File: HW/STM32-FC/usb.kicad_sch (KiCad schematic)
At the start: 14 parts, among them J2 USB_C_USB2.0_14P, J3 GH 1.25mm 6P, U2 USBLC6-2SC6, U3 AMS1117-3.3, U4 AMS1117-3.3

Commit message: 2025.02.07 USB C Conn change v1
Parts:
- C13, C14, C17, C18: LCSC C40894 -> C77000
- C15, C16: LCSC C1581 -> C1525
- J2: LCSC C5143397 -> C709031
- J3: LCSC C19626244 -> C133065
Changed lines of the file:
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@@
 			)
 		)
-		(property "LCSC" "C1581"
+		(property "LCSC" "C1525"
 			(at 171.45 35.56 0)
 			(effects
@@
 			)
 		)
-		(property "LCSC" "C40894"
+		(property "LCSC" "C77000"
 			(at 180.34 60.96 0)
 			(effects
@@
 			)
 		)
-		(property "LCSC" "C19626244 "
+		(property "LCSC" "C133065"
 			(at 229.87 35.56 0)
 			(effects
@@
 			)
 		)
-		(property "LCSC" "C40894"
+		(property "LCSC" "C77000"
 			(at 151.13 35.56 0)
 			(effects
@@
 			)
 		)
-		(property "LCSC" "C1581"
+		(property "LCSC" "C1525"
 			(at 171.45 60.96 0)
 			(effects
@@
 			)
 		)
-		(property "LCSC" "C40894"
+		(property "LCSC" "C77000"
 			(at 180.34 35.56 0)
 			(effects
@@
 			)
 		)
-		(property "LCSC" "C40894"
+		(property "LCSC" "C77000"
 			(at 151.13 60.96 0)
 			(effects
@@
 			)
 		)
-		(property "Datasheet" "https://www.usb.org/sites/default/files/documents/usb_type-c.zip"
+		(property "Datasheet" "~"
 			(at 49.53 46.99 0)
 			(effects
@@
 			)
 		)
-		(property "LCSC" "C5143397"
+		(property "LCSC" "C709031"
 			(at 45.72 46.99 0)
 			(effects

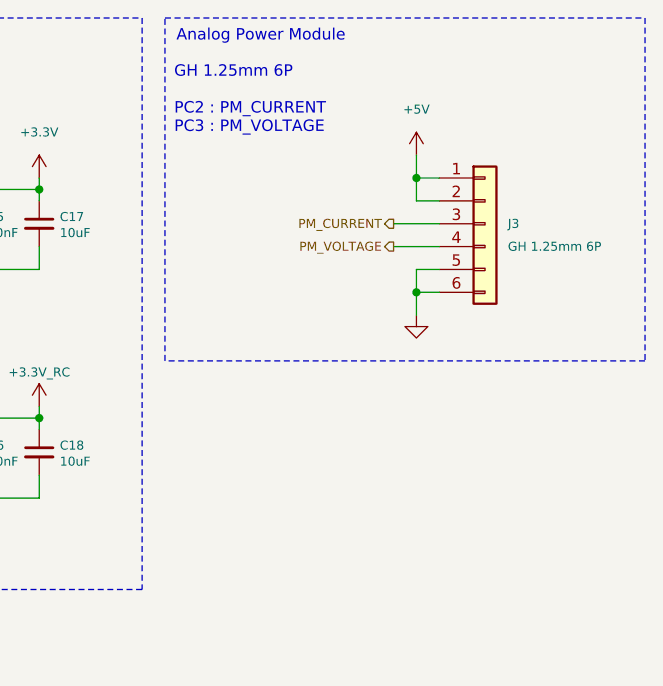
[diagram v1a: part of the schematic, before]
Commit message: 2025.02.11 PCB DONE! MEMO UPDATING
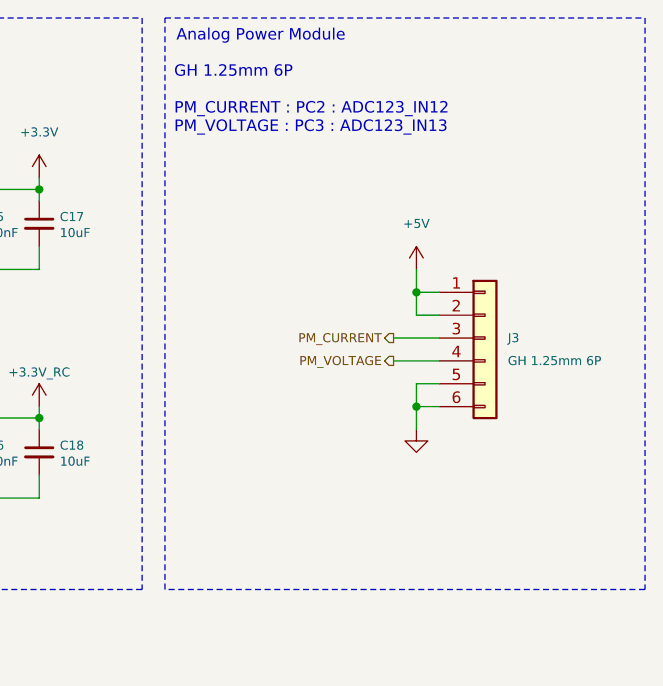
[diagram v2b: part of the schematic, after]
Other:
- note added: "GH 1.25mm 6P PM_CURRENT : PC2 : ADC123_IN12 PM_VOLTAGE : PC3 : ADC123_IN13"
- note removed: "GH 1.25mm 6P PC2 : PM_CURRENT PC3 : PM_VOLTAGE"
- moved on the sheet: J3
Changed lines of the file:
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@@
 	(title_block
 		(title "USB & POWER")
-		(date "2025-02-05")
+		(date "2025-02-08")
 		(rev "A")
 		(company "NARAE")
@@
 	)
 	(junction
-		(at 222.25 43.18)
+		(at 222.25 55.88)
 		(diameter 0)
 		(color 0 0 0 0)
@@
 	)
 	(junction
-		(at 222.25 30.48)
+		(at 222.25 43.18)
 		(diameter 0)
 		(color 0 0 0 0)
@@
 	(wire
 		(pts
-			(xy 222.25 30.48) (xy 222.25 33.02)
+			(xy 222.25 43.18) (xy 222.25 45.72)
 		)
 		(stroke
@@
 	(wire
 		(pts
-			(xy 219.71 35.56) (xy 224.79 35.56)
+			(xy 219.71 48.26) (xy 224.79 48.26)
 		)
 		(stroke
@@
 	(wire
 		(pts
-			(xy 224.79 40.64) (xy 222.25 40.64)
+			(xy 224.79 53.34) (xy 222.25 53.34)
 		)
 		(stroke
@@
 	(wire
 		(pts
-			(xy 222.25 43.18) (xy 222.25 45.72)
+			(xy 222.25 55.88) (xy 222.25 58.42)
 		)
 		(stroke
@@
 	(wire
 		(pts
-			(xy 222.25 40.64) (xy 222.25 43.18)
+			(xy 222.25 53.34) (xy 222.25 55.88)
 		)
 		(stroke
@@
 	(wire
 		(pts
-			(xy 222.25 27.94) (xy 222.25 30.48)
+			(xy 222.25 40.64) (xy 222.25 43.18)
 		)
 		(stroke
@@
 	(wire
 		(pts
-			(xy 224.79 43.18) (xy 222.25 43.18)
+			(xy 224.79 55.88) (xy 222.25 55.88)
 		)
 		(stroke
@@
 	(wire
 		(pts
-			(xy 224.79 33.02) (xy 222.25 33.02)
+			(xy 224.79 45.72) (xy 222.25 45.72)
 		)
 		(stroke
@@
 	(wire
 		(pts
-			(xy 219.71 38.1) (xy 224.79 38.1)
+			(xy 219.71 50.8) (xy 224.79 50.8)
 		)
 		(stroke
@@
 	(wire
 		(pts
-			(xy 222.25 30.48) (xy 224.79 30.48)
+			(xy 222.25 43.18) (xy 224.79 43.18)
 		)
 		(stroke
@@
 	(rectangle
 		(start 194.31 12.7)
-		(end 247.65 50.8)
+		(end 247.65 76.2)
 		(stroke
 			(width 0)
@@
 		)
 	)
-	(text "GH 1.25mm 6P\n\nPC2 : PM_CURRENT\nPC3 : PM_VOLTAGE"
+	(text "GH 1.25mm 6P\n\nPM_CURRENT : PC2 : ADC123_IN12\nPM_VOLTAGE : PC3 : ADC123_IN13"
 		(exclude_from_sim no)
 		(at 195.326 18.034 0)
@@
 	(hierarchical_label "PM_CURRENT"
 		(shape output)
-		(at 219.71 35.56 180)
+		(at 219.71 48.26 180)
 		(effects
 			(font
@@
 	(hierarchical_label "PM_VOLTAGE"
 		(shape output)
-		(at 219.71 38.1 180)
+		(at 219.71 50.8 180)
 		(effects
 			(font
@@
 	(symbol
 		(lib_id "power:+5V")
-		(at 222.25 27.94 0)
+		(at 222.25 40.64 0)
 		(unit 1)
 		(exclude_from_sim no)
@@
 		(fields_autoplaced yes)
 		(property "Reference" "#PWR039"
-			(at 222.25 31.75 0)
+			(at 222.25 44.45 0)
 			(effects
 				(font
@@
 		)
 		(property "Value" "+5V"
-			(at 222.25 22.86 0)
+			(at 222.25 35.56 0)
 			(effects
 				(font
@@
 		)
 		(property "Footprint" ""
-			(at 222.25 27.94 0)
+			(at 222.25 40.64 0)
 			(effects
 				(font
@@
 		)
 		(property "Datasheet" ""
-			(at 222.25 27.94 0)
+			(at 222.25 40.64 0)
 			(effects
 				(font
@@
 		)
 		(property "Description" "Power symbol creates a global label with name \"+5V\""
-			(at 222.25 27.94 0)
+			(at 222.25 40.64 0)
 			(effects
 				(font
@@
 	(symbol
 		(lib_id "Connector_Generic:Conn_01x06")
-		(at 229.87 35.56 0)
+		(at 229.87 48.26 0)
 		(unit 1)
 		(exclude_from_sim no)
@@
 		(dnp no)
 		(property "Reference" "J3"
-			(at 232.41 35.56 0)
+			(at 232.41 48.26 0)
 			(effects
 				(font
@@
 		)
 		(property "Value" "GH 1.25mm 6P"
-			(at 232.41 38.1 0)
+			(at 232.41 50.8 0)
 			(effects
 				(font
@@
 		)
 		(property "Footprint" "JST_GH:JST_GH_SM06B-GHS-TB_06x1.25mm_Angled"
-			(at 229.87 35.56 0)
+			(at 229.87 48.26 0)
 			(effects
 				(font
@@
 		)
 		(property "Datasheet" "~"
-			(at 229.87 35.56 0)
+			(at 229.87 48.26 0)
 			(effects
 				(font
@@
 		)
 		(property "Description" "Generic connector, single row, 01x06, script generated (kicad-library-utils/schlib/autogen/connector/)"
-			(at 229.87 35.56 0)
+			(at 229.87 48.26 0)
 			(effects
 				(font
@@
 		)
 		(property "Availability" ""
-			(at 229.87 35.56 0)
+			(at 229.87 48.26 0)
 			(effects
 				(font
@@
 		)
 		(property "Check_prices" ""
-			(at 229.87 35.56 0)
+			(at 229.87 48.26 0)
 			(effects
 				(font
@@
 		)
 		(property "Description_1" ""
-			(at 229.87 35.56 0)
+			(at 229.87 48.26 0)
 			(effects
 				(font
@@
 		)
 		(property "MF" ""
-			(at 229.87 35.56 0)
+			(at 229.87 48.26 0)
 			(effects
 				(font
@@
 		)
 		(property "MP" ""
-			(at 229.87 35.56 0)
+			(at 229.87 48.26 0)
 			(effects
 				(font
@@
 		)
 		(property "Package" ""
-			(at 229.87 35.56 0)
+			(at 229.87 48.26 0)
 			(effects
 				(font
@@
 		)
 		(property "Price" ""
-			(at 229.87 35.56 0)
+			(at 229.87 48.26 0)
 			(effects
 				(font
@@
 		)
 		(property "SnapEDA_Link" ""
-			(at 229.87 35.56 0)
+			(at 229.87 48.26 0)
 			(effects
 				(font
@@
 		)
 		(property "Sim.Device" ""
-			(at 229.87 35.56 0)
+			(at 229.87 48.26 0)
 			(effects
 				(font
@@
 		)
 		(property "Sim.Pins" ""
-			(at 229.87 35.56 0)
+			(at 229.87 48.26 0)
 			(effects
 				(font
@@
 		)
 		(property "LCSC" "C133065"
-			(at 229.87 35.56 0)
+			(at 229.87 48.26 0)
 			(effects
 				(font
@@
 		)
 		(property "JLC" ""
-			(at 229.87 35.56 0)
+			(at 229.87 48.26 0)
 			(effects
 				(font
@@
 	(symbol
 		(lib_id "power:GND")
-		(at 222.25 45.72 0)
+		(at 222.25 58.42 0)
 		(unit 1)
 		(exclude_from_sim no)
@@
 		(fields_autoplaced yes)
 		(property "Reference" "#PWR040"
-			(at 222.25 52.07 0)
+			(at 222.25 64.77 0)
 			(effects
 				(font
@@
 		)
 		(property "Value" "GND"
-			(at 222.25 50.8 0)
+			(at 222.25 63.5 0)
 			(effects
 				(font
@@
 		)
 		(property "Footprint" ""
-			(at 222.25 45.72 0)
+			(at 222.25 58.42 0)
 			(effects
 				(font
@@
 		)
 		(property "Datasheet" ""
-			(at 222.25 45.72 0)
+			(at 222.25 58.42 0)
 			(effects
 				(font
@@
 		)
 		(property "Description" "Power symbol creates a global label with name \"GND\" , ground"
-			(at 222.25 45.72 0)
+			(at 222.25 58.42 0)
 			(effects
 				(font
